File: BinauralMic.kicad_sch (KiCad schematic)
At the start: 0 parts

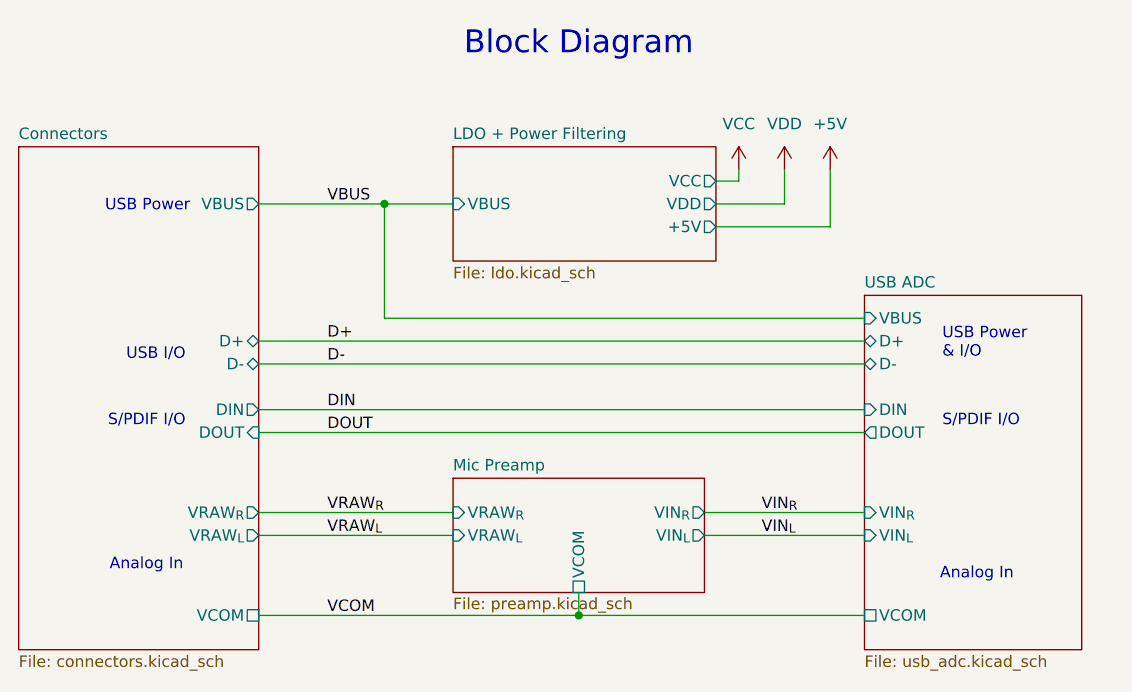
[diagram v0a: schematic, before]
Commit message: Resnap text to grid + add .gitignore
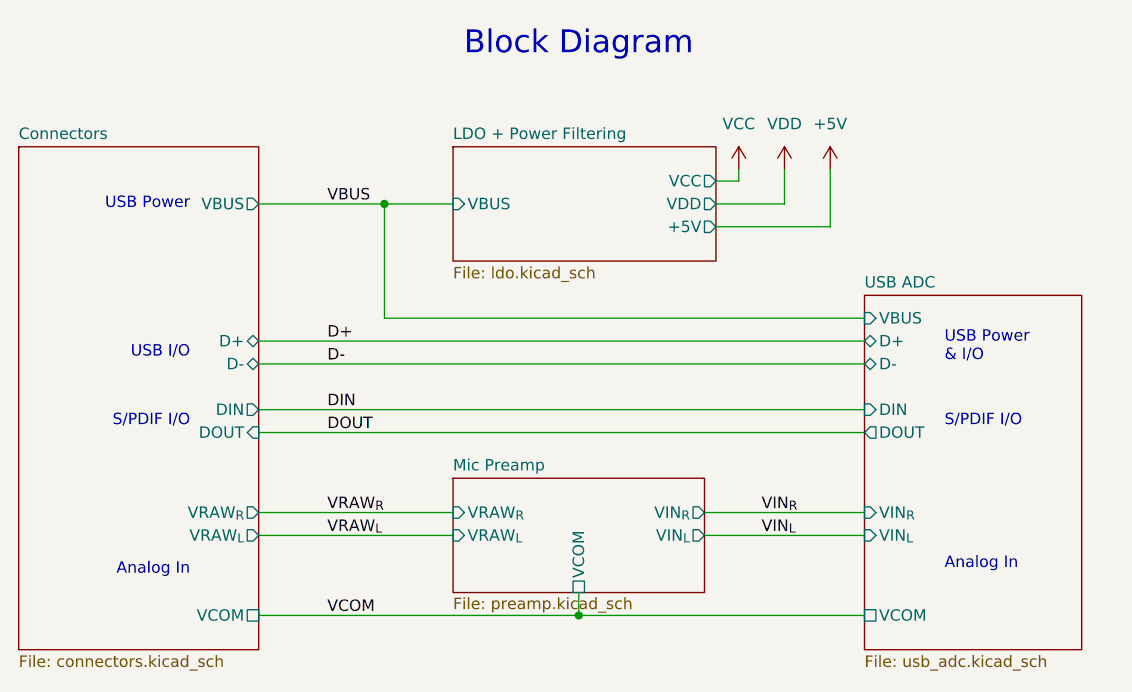
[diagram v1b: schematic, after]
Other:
- title: Binaural Mic -> Binaural Mic (Block Diagram)
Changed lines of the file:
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@@
 	(paper "A5")
 	(title_block
-		(title "Binaural Mic")
-		(date "2024-09-12")
+		(title "Binaural Mic (Block Diagram)")
+		(date "2024-09-15")
 		(rev "1")
 		(company "Tachyon PCBAs")
@@
 	(text "Analog In"
 		(exclude_from_sim no)
-		(at 144.272 85.598 0)
+		(at 144.78 84.455 0)
 		(effects
 			(font
@@
 	(text "USB Power"
 		(exclude_from_sim no)
-		(at 60.96 44.704 0)
+		(at 60.96 44.45 0)
 		(effects
 			(font
@@
 	(text "S/PDIF I/O"
 		(exclude_from_sim no)
-		(at 144.526 68.58 0)
+		(at 144.78 68.58 0)
 		(effects
 			(font
@@
 	(text "USB I/O"
 		(exclude_from_sim no)
-		(at 60.452 61.214 0)
+		(at 60.96 60.96 0)
 		(effects
 			(font
@@
 	(text "USB Power\n& I/O"
 		(exclude_from_sim no)
-		(at 144.526 59.944 0)
+		(at 144.78 60.325 0)
 		(effects
 			(font
@@
 	(text "S/PDIF I/O"
 		(exclude_from_sim no)
-		(at 60.452 68.58 0)
+		(at 60.96 68.58 0)
 		(effects
 			(font
@@
 	(text "Analog In"
 		(exclude_from_sim no)
-		(at 60.198 84.582 0)
-		(effects
-			(font
+		(at 60.96 85.09 0)
+		(effects
+			(font
